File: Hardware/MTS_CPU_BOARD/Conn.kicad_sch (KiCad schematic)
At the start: 8 parts, among them J1 DIN41612_02x16_ZB, SW1 SW_DIP_x04, U1 TCAN337GDR, U3 24LC32

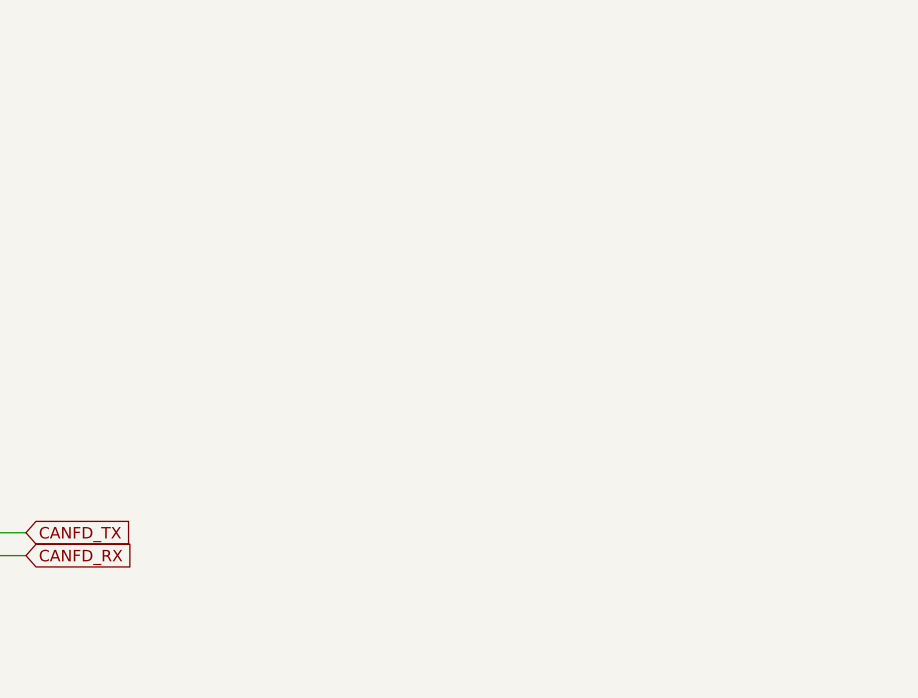
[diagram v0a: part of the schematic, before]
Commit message: Add some connectors
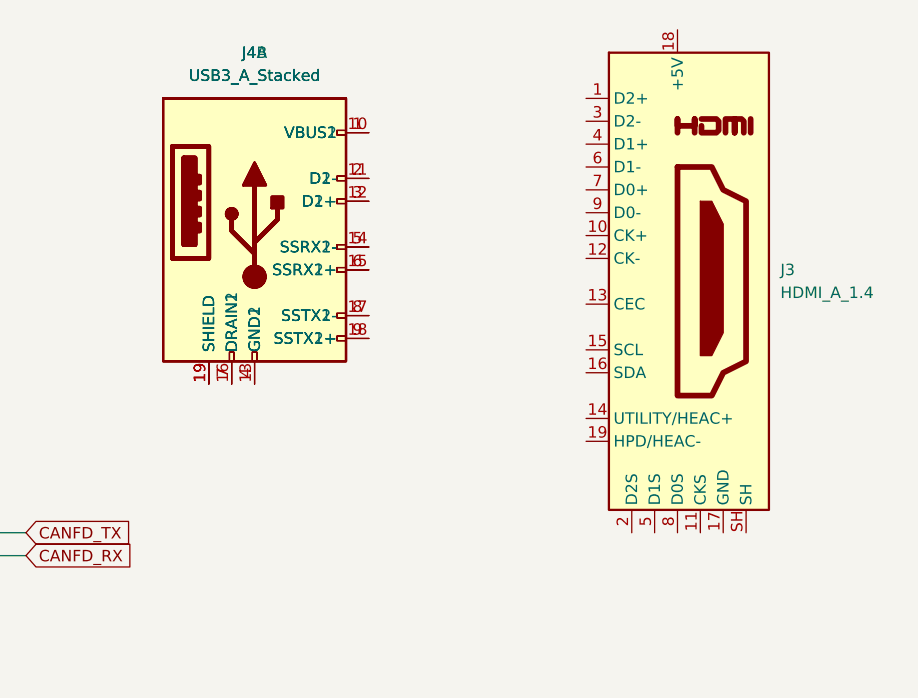
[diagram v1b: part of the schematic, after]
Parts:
- added J3: HDMI_A_1.4, Connector_Video:HDMI_A_Kycon_KDMIX-SL1-NS-WS-B15_VerticalRightAngle, symbol Connector:HDMI_A_1.4
- added J4: USB3_A_Stacked, Connector_USB:USB3_A_Molex_48406-0001_Horizontal_Stacked, symbol Connector:USB3_A_Stacked
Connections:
- new net: J4.1 (VBUS1), J4.10 (VBUS2)
- new net: J4.19 (SHIELD), J4.19 (SHIELD)
- new net: J4.11 (D2-), J4.2 (D1-)
- new net: J4.12 (D2+), J4.3 (D1+)
- new net: J4.13 (GND2), J4.4 (GND1)
- new net: J4.14 (SSRX2-), J4.5 (SSRX1-)
- new net: J4.15 (SSRX2+), J4.6 (SSRX1+)
- new net: J4.16 (DRAIN2), J4.7 (DRAIN1)
- new net: J4.17 (SSTX2-), J4.8 (SSTX1-)
- new net: J4.18 (SSTX2+), J4.9 (SSTX1+)
